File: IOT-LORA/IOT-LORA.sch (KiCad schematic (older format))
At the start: 36 parts, among them J1 Conn_01x02, J2 Conn_01x06, J3 Conn_01x03, J4 Conn_01x03, J5 Conn_01x03, J6 Conn_01x03, J7 Conn_01x04, J8 Conn_01x04, J9 Conn_01x06, U1 LM1117-3.3, U2 ATmega328-AU, U3 Ai-Thinker-Ra-01, Y1 Crystal_Small

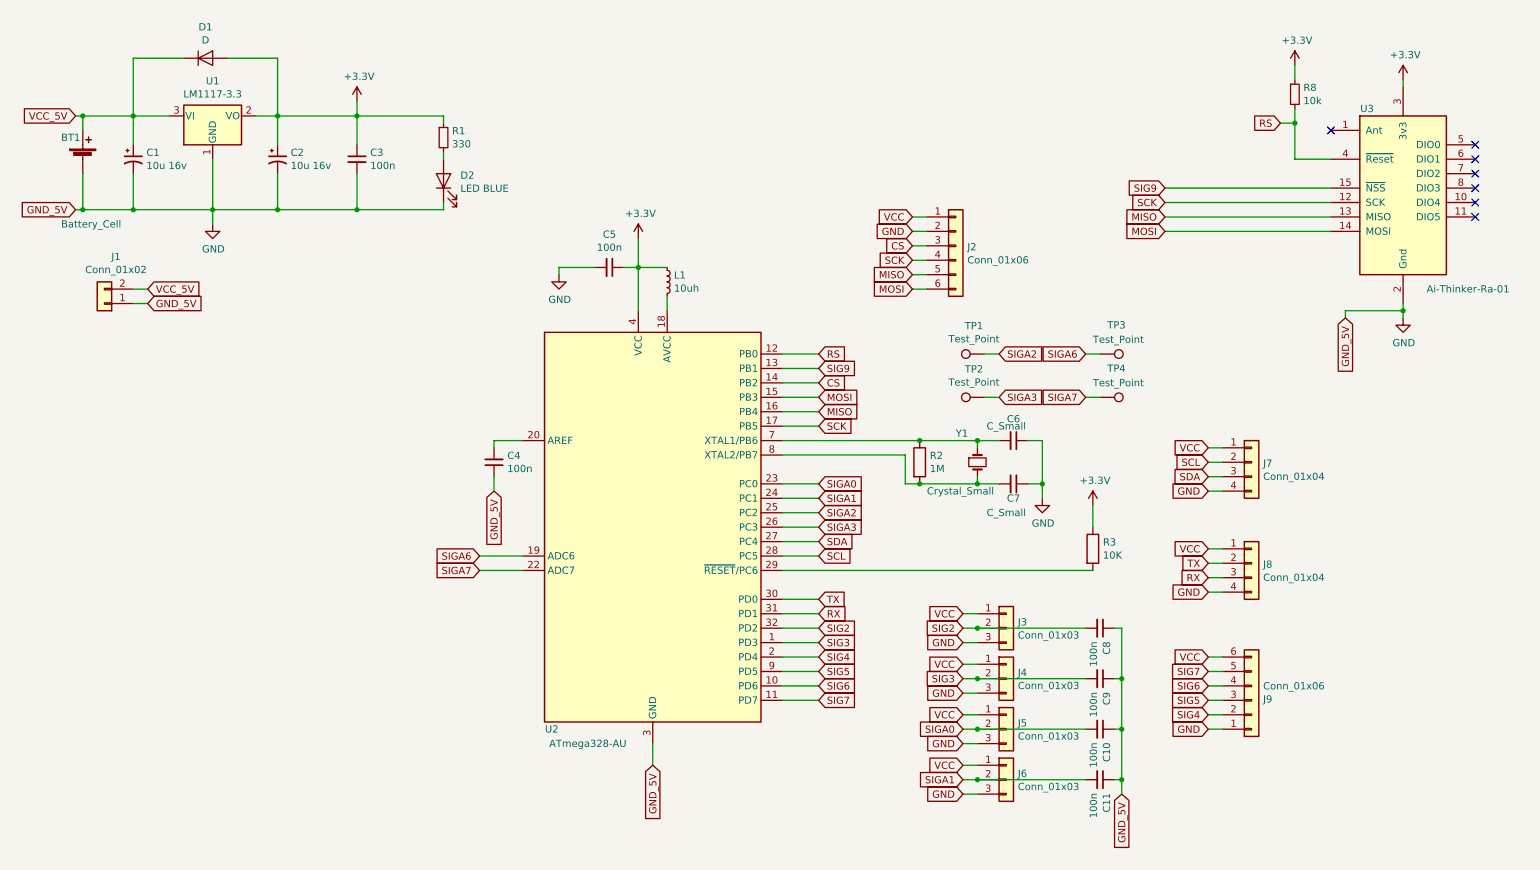
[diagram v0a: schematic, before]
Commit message: modifier
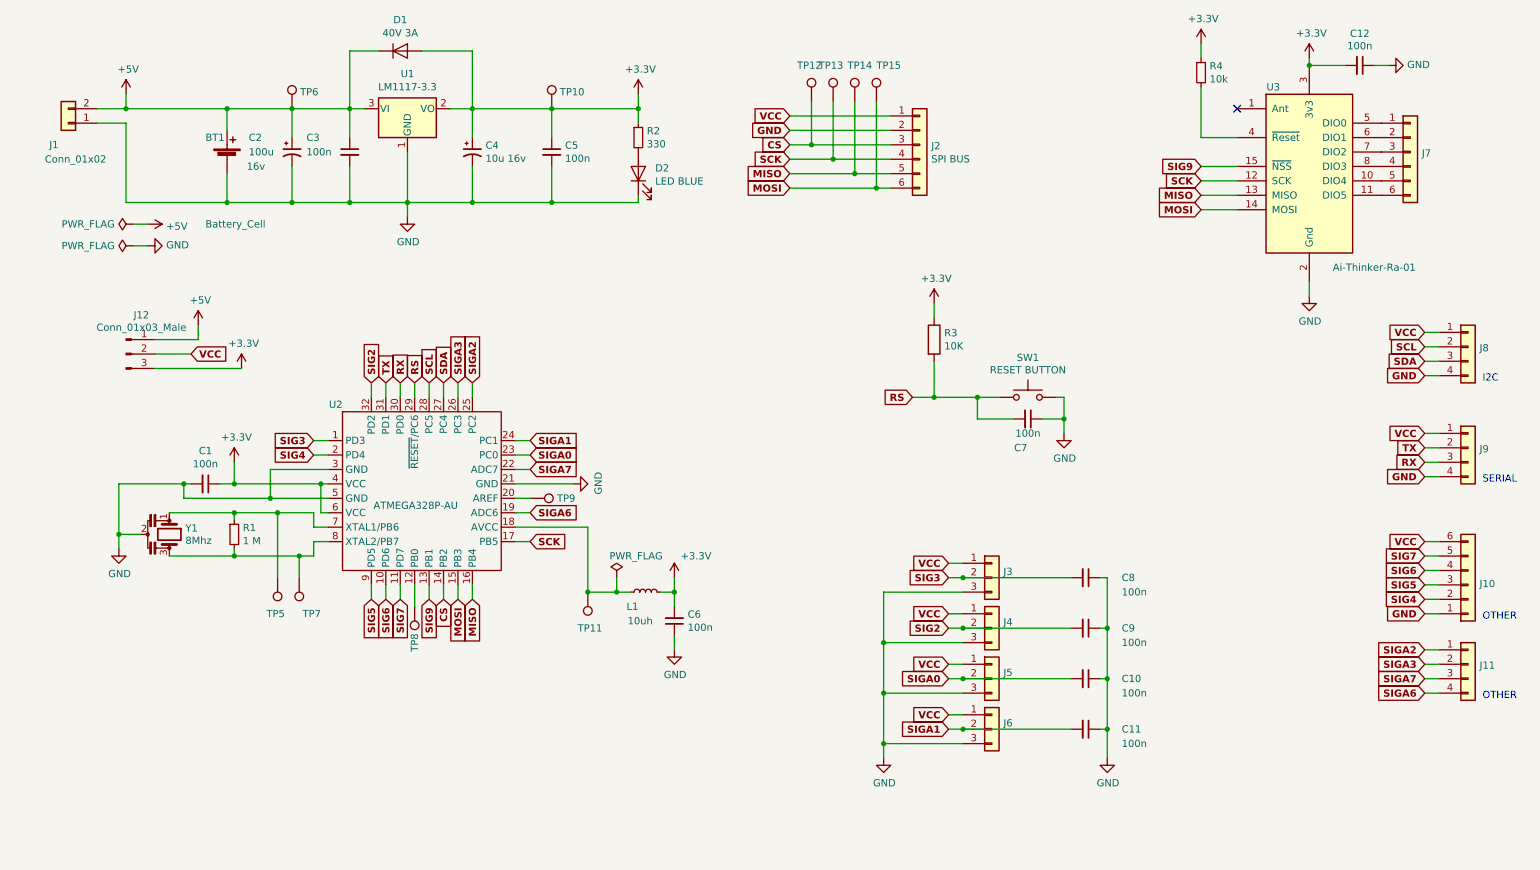
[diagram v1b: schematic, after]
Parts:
- removed C6: C_Small, Capacitor_SMD:C_0805_2012Metric_Pad1.15x1.50mm_HandSolder, symbol Device:C_Small
- removed R2: 1M, Resistor_SMD:R_0603_1608Metric_Pad0.84x1.00mm_HandSolder, symbol Device:R
- removed TP1, TP2, TP3, TP4: Test_Point, TestPoint:TestPoint_Pad_D1.0mm, symbol Connector_Specialized:Test_Point
- removed U2: ATmega328-AU, Package_QFP:TQFP-32_7x7mm_P0.8mm, symbol MCU_Microchip_ATmega:ATmega328-AU
- removed Y1: Crystal_Small, Crystal:Crystal_SMD_HC49-SD_HandSoldering, symbol Device:Crystal_Small
- added C12, C3: 100n, LEEVAWN:C_0603_1608Metric_Pad0.84x1.00mm_HandSolder_jp, symbol Device:C_Small
- added J11: Conn_01x04, Connector_PinSocket_2.54mm:PinSocket_1x04_P2.54mm_Vertical, symbol Connector_Generic:Conn_01x04
- added J12: Conn_01x03_Male, Connector_PinHeader_2.54mm:PinHeader_1x03_P2.54mm_Vertical, symbol Connector:Conn_01x03_Male
- added J7: Conn_01x06, Connector_PinSocket_2.54mm:PinSocket_1x06_P2.54mm_Vertical, symbol Connector_Generic:Conn_01x06
- added R1: 1 M, LEEVAWN:R_0805_2012Metric_jp, symbol Device:R_Small
- added SW1: RESET BUTTON, LEEVAWN:EL-3625-W, symbol Switch:SW_Push
- added TP10, TP11, TP12, TP13, TP14, TP15, TP5, TP6, TP7: TestPoint, TestPoint:TestPoint_Pad_D1.0mm, symbol Connector:TestPoint
- added TP8, TP9: Test_Point, TestPoint:TestPoint_Pad_D1.0mm, symbol IOT-LORA-rescue:Test_Point-Connector_Specialized
- added U2: ATMEGA328P-AU, Package_QFP:TQFP-32_7x7mm_P0.8mm, symbol LEEVAWNS:ATMEGA328P-AU
- added Y1: 8Mhz, LEEVAWN:CSTNE16M00V2, symbol Device:Resonator
- C1: renamed from C5; footprint Capacitor_SMD:C_0805_2012Metric_Pad1.15x1.50mm_HandSolder -> LEEVAWN:C_0603_1608Metric_Pad0.84x1.00mm_HandSolder_jp
- C10, C11, C8, C9: footprint Capacitor_SMD:C_0805_2012Metric_Pad1.15x1.50mm_HandSolder -> LEEVAWN:C_0603_1608Metric_Pad0.84x1.00mm_HandSolder_jp
- C2: renamed from C1; value 10u 16v -> 100u; footprint Capacitor_SMD:CP_Elec_4x5.3 -> LEEVAWN:CP_Elec_6.3x7.7_jp; Field4 (none) -> 16v
- C4: renamed from C2; footprint Capacitor_SMD:CP_Elec_4x5.3 -> LEEVAWN:CP_Elec_4x5.3_jp
- C5: renamed from C3; footprint Capacitor_SMD:C_0805_2012Metric_Pad1.15x1.50mm_HandSolder -> LEEVAWN:C_0603_1608Metric_Pad0.84x1.00mm_HandSolder_jp
- C6: renamed from C4; footprint Capacitor_SMD:C_0805_2012Metric_Pad1.15x1.50mm_HandSolder -> LEEVAWN:C_0603_1608Metric_Pad0.84x1.00mm_HandSolder_jp
- C7: value C_Small -> 100n; footprint Capacitor_SMD:C_0805_2012Metric_Pad1.15x1.50mm_HandSolder -> LEEVAWN:C_0603_1608Metric_Pad0.84x1.00mm_HandSolder_jp
- D1: value D -> 40V 3A; footprint Diode_SMD:D_SMA -> LEEVAWN:D_SMA
- D2: footprint LED_SMD:LED_0805_2012Metric_Pad0.97x1.50mm_HandSolder -> LEEVAWN:LED_0805_2012Metric_Pad0.97x1.50mm_HandSolder
- J1: footprint Connector_JST:JST_XH_B02B-XH-A_1x02_P2.50mm_Vertical -> LEEVAWN:2P-XH2.54-V
- J10: renamed from J9; footprint Connector_JST:JST_XH_B06B-XH-A_1x06_P2.50mm_Vertical -> Connector_PinSocket_2.54mm:PinSocket_1x06_P2.54mm_Vertical
- J2: value Conn_01x06 -> SPI BUS; footprint Connector_JST:JST_XH_B06B-XH-A_1x06_P2.50mm_Vertical -> Connector_PinSocket_2.54mm:PinSocket_1x06_P2.54mm_Vertical
- J3, J4, J5, J6: footprint Connector_JST:JST_XH_B03B-XH-A_1x03_P2.50mm_Vertical -> LEEVAWN:3P-XH2.54-V
- J8: renamed from J7; footprint Connector_JST:JST_XH_B04B-XH-A_1x04_P2.50mm_Vertical -> Connector_PinSocket_2.54mm:PinSocket_1x04_P2.54mm_Vertical
- J9: renamed from J8; footprint Connector_JST:JST_XH_B04B-XH-A_1x04_P2.50mm_Vertical -> Connector_PinSocket_2.54mm:PinSocket_1x04_P2.54mm_Vertical
- R2: renamed from R1; footprint Resistor_SMD:R_0805_2012Metric_Pad1.15x1.50mm_HandSolder -> LEEVAWN:R_0603_1608Metric_Pad0.84x1.00mm_HandSolder_jp
- R3: footprint Resistor_SMD:R_0805_2012Metric_Pad1.15x1.50mm_HandSolder -> LEEVAWN:R_0603_1608Metric_Pad0.84x1.00mm_HandSolder_jp
- R4: renamed from R8; footprint Resistor_SMD:R_0805_2012Metric_Pad1.15x1.50mm_HandSolder -> LEEVAWN:R_0603_1608Metric_Pad0.84x1.00mm_HandSolder_jp
- U1: footprint Package_TO_SOT_SMD:SOT-223-3_TabPin2 -> LEEVAWN:SOT-223-3_TabPin2
- U3: footprint RF_Module:Ai-Thinker-Ra-01-LoRa -> LEEVAWN:Ai-Thinker-Ra-01-LoRa
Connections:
- net +3V3: now also C6.2, L1.2, C12.2, J12.3 (Pin_3), TP10.1, U2.4 (VCC), U2.6 (VCC); no longer L1.1
- net CS: now also TP12.1, U2.14 (PB2)
- net GND: now also C12.1, C3.2, SW1.2, U2.3 (GND), U2.5 (GND), Y1.2
- net MISO: now also TP14.1, U2.16 (PB4)
- net MOSI: now also TP15.1, U2.15 (PB3)
- net RS: now also C7.2, R3.2, SW1.1, U2.29 (~RESET~/PC6); no longer R4.2, U3.4 (~Reset)
- net RX: now also U2.30 (PD0)
- net SCK: now also TP13.1, U2.17 (PB5)
- net SCL: now also U2.28 (PC5)
- net SDA: now also U2.27 (PC4)
- net SIG2: now also C9.2, J4.2 (Pin_2), U2.32 (PD2); no longer C8.2, J3.2 (Pin_2)
- net SIG3: now also C8.2, J3.2 (Pin_2), U2.1 (PD3); no longer C9.2, J4.2 (Pin_2)
- net SIG4: now also U2.2 (PD4)
- net SIG5: now also U2.9 (PD5)
- net SIG6: now also U2.10 (PD6)
- net SIG7: now also U2.11 (PD7)
- net SIG9: now also U2.13 (PB1)
- net SIGA0: now also U2.23 (PC0)
- net SIGA1: now also U2.24 (PC1)
- net SIGA2: now also J11.1 (Pin_1), U2.25 (PC2)
- net SIGA3: now also J11.2 (Pin_2), U2.26 (PC3)
- net SIGA6: now also J11.4 (Pin_4), U2.19 (ADC6)
- net SIGA7: now also J11.3 (Pin_3), U2.22 (ADC7)
- net TX: now also U2.31 (PD1)
- net VCC: now also J12.2 (Pin_2)
- net at U3.10 (DIO4): now also J7.5 (Pin_5)
- net at U3.11 (DIO5): now also J7.6 (Pin_6)
- net at U3.5 (DIO0): now also J7.1 (Pin_1)
- net at U3.6 (DIO1): now also J7.2 (Pin_2)
- net at U3.7 (DIO2): now also J7.3 (Pin_3)
- net at U3.8 (DIO3): now also J7.4 (Pin_4)
- net VCC_5V renamed +5V
- net +5V: now also C3.1, J12.1 (Pin_1), TP6.1
- new net: R4.2, U3.4 (~Reset)
- new net: L1.1, TP11.1, U2.18 (AVCC)
- new net: TP8.1, U2.12 (PB0)
- new net: TP9.1, U2.20 (AREF)
- new net: R1.1, TP5.1, U2.7 (XTAL1/PB6), Y1.1
- new net: R1.2, TP7.1, U2.8 (XTAL2/PB7), Y1.3
- no-connect marks 7 -> 1
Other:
- note added: "I2C"
- note added: "OTHER"
- note added: "SERIAL"
- moved on the sheet: BT1, C1, C10, C11, C2, C4, C5, C6, C8, C9, D1, D2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
